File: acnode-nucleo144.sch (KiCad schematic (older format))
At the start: 9 parts, among them J1 8P8C_Shielded, J2 8P8C_Shielded, U1 ISL3176EIBZ, U2 Nucleo-144, U3 W25Q32JVSS

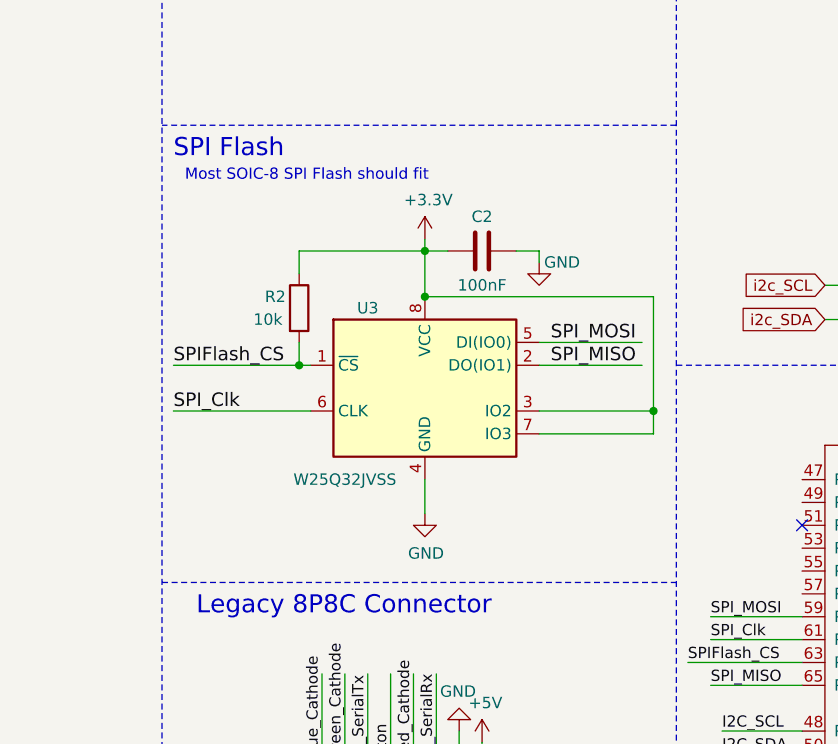
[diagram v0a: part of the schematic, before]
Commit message: Some changes I found on my computer
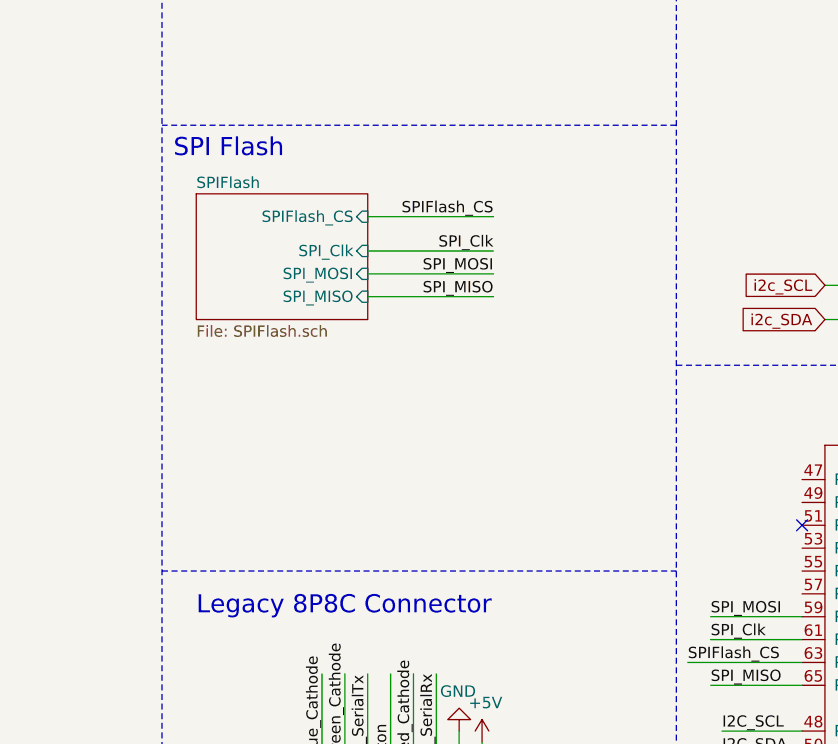
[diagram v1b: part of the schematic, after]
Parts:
- removed C2: 100nF, Capacitor_SMD:C_0603_1608Metric, symbol Device:C
- removed R2: 10k, Resistor_SMD:R_0603_1608Metric, symbol Device:R
- removed U3: W25Q32JVSS, Package_SO:SOIC-8_5.23x5.23mm_P1.27mm, symbol Memory_Flash:W25Q32JVSS
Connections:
- wire segments 108 -> 93
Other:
- note removed: "Most SOIC-8 SPI Flash should fit"
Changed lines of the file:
@@
 $Descr A4 11693 8268
 encoding utf-8
-Sheet 1 4
+Sheet 1 5
 Title "ACNode Nucleo-144 Overlay"
 Date "2020-11-28"
@@
 Text Notes 3400 6050 0    79   ~ 0
 Legacy 8P8C Connector
-$Comp
-L Memory_Flash:W25Q32JVSS U3
-U 1 1 5FD27D8E
-P 4400 5050
-F 0 "U3" H 4150 5400 50  0000 C CNN
-F 1 "W25Q32JVSS" H 4050 4650 50  0000 C CNN
-F 2 "Package_SO:SOIC-8_5.23x5.23mm_P1.27mm" H 4400 5050 50  0001 C CNN
-F 3 "http://www.winbond.com/resource-files/w25q32jv%20revg%2003272018%20plus.pdf" H 4400 5050 50  0001 C CNN
-	1    4400 5050
-	1    0    0    -1
-$EndComp
-$Comp
-L power:GND #PWR0108
-U 1 1 5FD2EDFB
-P 4400 5600
-F 0 "#PWR0108" H 4400 5350 50  0001 C CNN
-F 1 "GND" H 4405 5427 50  0000 C CNN
-F 2 "" H 4400 5600 50  0001 C CNN
-F 3 "" H 4400 5600 50  0001 C CNN
-	1    4400 5600
-	1    0    0    -1
-$EndComp
-Wire Wire Line
-	4400 4650 4400 4450
-Wire Wire Line
-	4400 5600 4400 5450
-$Comp
-L Device:C C2
-U 1 1 5FD31B13
-P 4650 4450
-F 0 "C2" V 4500 4450 50  0000 C CNN
-F 1 "100nF" V 4800 4450 50  0000 C CNN
-F 2 "Capacitor_SMD:C_0603_1608Metric" H 4688 4300 50  0001 C CNN
-F 3 "~" H 4650 4450 50  0001 C CNN
-	1    4650 4450
-	0    1    1    0
-$EndComp
-Wire Wire Line
-	4500 4450 4400 4450
-Connection ~ 4400 4450
-Wire Wire Line
-	4400 4450 4400 4400
-Wire Wire Line
-	4800 4450 4900 4450
-$Comp
-L power:+3.3V #PWR0110
-U 1 1 5FD34D1D
-P 4400 4400
-F 0 "#PWR0110" H 4400 4250 50  0001 C CNN
-F 1 "+3.3V" H 4415 4573 50  0000 C CNN
-F 2 "" H 4400 4400 50  0001 C CNN
-F 3 "" H 4400 4400 50  0001 C CNN
-	1    4400 4400
-	1    0    0    -1
-$EndComp
-Text Label 3300 4950 0    59   ~ 0
-SPIFlash_CS
-Wire Wire Line
-	3900 4950 3850 4950
-Wire Wire Line
-	3900 5150 3300 5150
-Text Label 3300 5150 0    59   ~ 0
-SPI_Clk
-Text Label 4950 4850 0    59   ~ 0
-SPI_MOSI
-Text Label 4950 4950 0    59   ~ 0
-SPI_MISO
-Wire Wire Line
-	4900 4500 4900 4450
 Text Notes 3300 4050 0    79   ~ 0
 SPI Flash
-Wire Wire Line
-	4900 4850 5350 4850
-Wire Wire Line
-	4900 4950 5350 4950
-Wire Wire Line
-	4900 5150 5400 5150
-Wire Wire Line
-	5400 5150 5400 4650
-Wire Wire Line
-	5400 4650 4400 4650
-Connection ~ 4400 4650
-Wire Wire Line
-	4900 5250 5400 5250
-Wire Wire Line
-	5400 5250 5400 5150
-Connection ~ 5400 5150
 Wire Notes Line
 	5500 3900 3250 3900
-Wire Notes Line
-	3250 5900 5500 5900
-$Comp
-L Device:R R2
-U 1 1 5FDA2BE7
-P 3850 4700
-F 0 "R2" H 3700 4750 50  0000 L CNN
-F 1 "10k" H 3650 4650 50  0000 L CNN
-F 2 "Resistor_SMD:R_0603_1608Metric" V 3780 4700 50  0001 C CNN
-F 3 "~" H 3850 4700 50  0001 C CNN
-	1    3850 4700
-	1    0    0    -1
-$EndComp
-Wire Wire Line
-	3850 4950 3850 4850
-Connection ~ 3850 4950
-Wire Wire Line
-	3850 4950 3300 4950
-Wire Wire Line
-	3850 4550 3850 4450
-Wire Wire Line
-	3850 4450 4400 4450
-Text Notes 3350 4150 0    49   ~ 0
-Most SOIC-8 SPI Flash should fit
 $Comp
 L ExtraParts:ISL8489EIBZ U1
@@
 	7050 700  7050 750
 $Comp
-L power:GND #PWR?
+L power:GND #PWR0108
 U 1 1 6036D39A
 P 7250 700
-F 0 "#PWR?" H 7250 450 50  0001 C CNN
+F 0 "#PWR0108" H 7250 450 50  0001 C CNN
 F 1 "GND" H 7255 527 50  0000 C CNN
 F 2 "" H 7250 700 50  0001 C CNN
@@
 $Comp
 L power:GND #PWR0109
-U 1 1 5FD2F252
-P 4900 4500
-F 0 "#PWR0109" H 4900 4250 50  0001 C CNN
-F 1 "GND" H 5000 4500 50  0000 C CNN
-F 2 "" H 4900 4500 50  0001 C CNN
-F 3 "" H 4900 4500 50  0001 C CNN
-	1    4900 4500
-	1    0    0    -1
-$EndComp
-$Comp
-L power:GND #PWR?
 U 1 1 6037908D
 P 4950 7400
-F 0 "#PWR?" H 4950 7150 50  0001 C CNN
+F 0 "#PWR0109" H 4950 7150 50  0001 C CNN
 F 1 "GND" H 4955 7227 50  0000 C CNN
 F 2 "" H 4950 7400 50  0001 C CNN
@@
 	1    0    0    -1
 $EndComp
+$Sheet
+S 3400 4200 750  550
+U 603F3E51
+F0 "SPIFlash" 49
+F1 "SPIFlash.sch" 49
+F2 "SPIFlash_CS" I R 4150 4300 49
+F3 "SPI_Clk" I R 4150 4450 49
+F4 "SPI_MOSI" I R 4150 4550 49
+F5 "SPI_MISO" I R 4150 4650 49
+$EndSheet
+Wire Notes Line
+	3250 5850 5500 5850
+Text Label 4700 4300 2    49   ~ 0
+SPIFlash_CS
+Text Label 4700 4450 2    49   ~ 0
+SPI_Clk
+Text Label 4700 4550 2    49   ~ 0
+SPI_MOSI
+Text Label 4700 4650 2    49   ~ 0
+SPI_MISO
+Wire Wire Line
+	4150 4300 4700 4300
+Wire Wire Line
+	4700 4450 4150 4450
+Wire Wire Line
+	4150 4550 4700 4550
+Wire Wire Line
+	4700 4650 4150 4650
 $EndSCHEMATC
